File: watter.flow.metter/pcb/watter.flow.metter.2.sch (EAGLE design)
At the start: 19 parts, among them Q1 BC546A

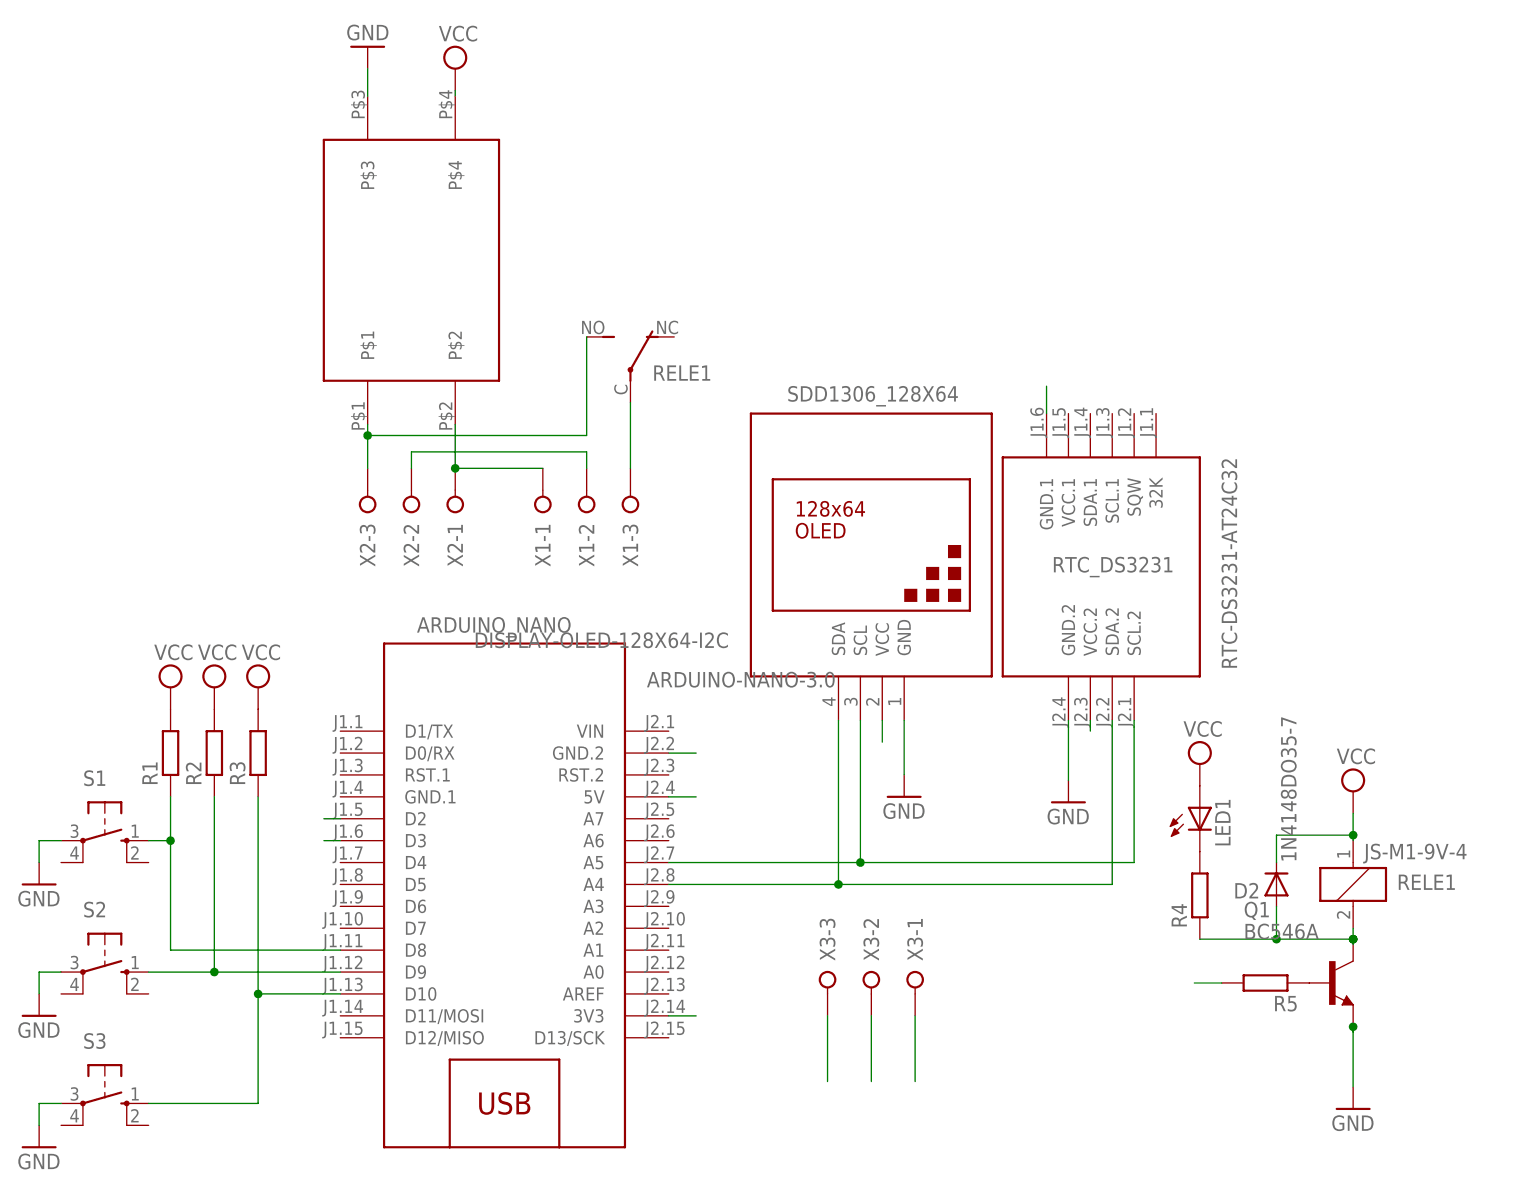
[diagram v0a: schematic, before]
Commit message: add terminal
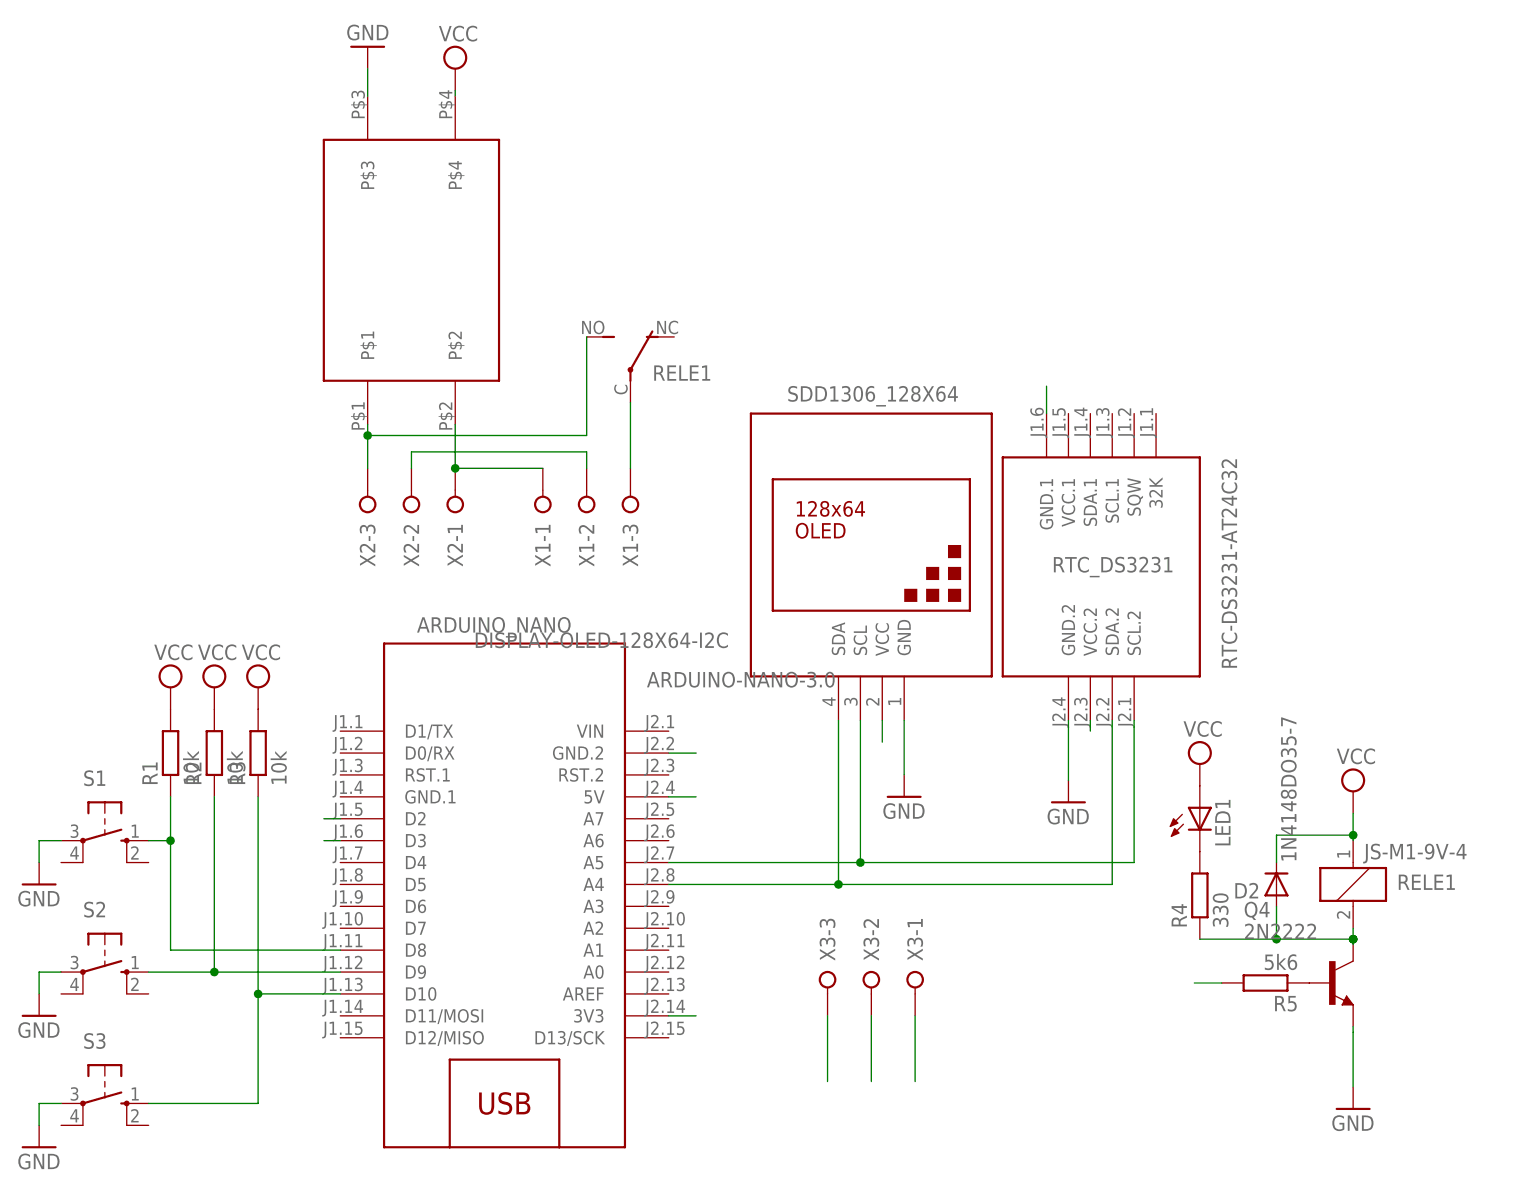
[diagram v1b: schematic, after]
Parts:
- removed Q1: BC546A, transistor-npn:BC546A
- added Q4: 2N2222, transistor-npn:2N5088
- R1, R2, R3: value (none) -> 10k
- R4: value (none) -> 330
- R5: value (none) -> 5k6
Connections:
- net GND: now also Q4.E; no longer Q1.E
- net N$41: now also Q4.C; no longer Q1.C
- net N$7: now also Q4.B; no longer Q1.B
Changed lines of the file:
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@@
 <?xml version="1.0" encoding="utf-8"?>
 <!DOCTYPE eagle SYSTEM "eagle.dtd">
-<eagle version="8.2.2">
+<eagle version="8.4.1">
 <drawing>
 <settings>
 <setting alwaysvectorfont="no"/>
+<setting keepoldvectorfont="yes"/>
 <setting verticaltext="up"/>
 </settings>
-<grid distance="0.1" unitdist="inch" unit="inch" style="lines" multiple="1" display="no" altdistance="0.01" altunitdist="inch" altunit="inch"/>
+<grid distance="0.05" unitdist="inch" unit="inch" style="lines" multiple="1" display="no" altdistance="0.01" altunitdist="inch" altunit="inch"/>
 <layers>
 <layer number="1" name="Top" color="4" fill="1" visible="no" active="no"/>
@@
 <part name="SUPPLY4" library="supply2" library_urn="urn:adsk.eagle:library:372" deviceset="VCC" device=""/>
 <part name="SUPPLY6" library="supply2" library_urn="urn:adsk.eagle:library:372" deviceset="VCC" device=""/>
-<part name="R1" library="rcl" library_urn="urn:adsk.eagle:library:334" deviceset="R-EU_" device="0207/10"/>
-<part name="R2" library="rcl" library_urn="urn:adsk.eagle:library:334" deviceset="R-EU_" device="0207/10"/>
-<part name="R3" library="rcl" library_urn="urn:adsk.eagle:library:334" deviceset="R-EU_" device="0207/10"/>
-<part name="Q1" library="transistor-npn" library_urn="urn:adsk.eagle:library:398" deviceset="BC546*" device="" technology="A"/>
+<part name="R1" library="rcl" library_urn="urn:adsk.eagle:library:334" deviceset="R-EU_" device="0207/10" value="10k"/>
+<part name="R2" library="rcl" library_urn="urn:adsk.eagle:library:334" deviceset="R-EU_" device="0207/10" value="10k"/>
+<part name="R3" library="rcl" library_urn="urn:adsk.eagle:library:334" deviceset="R-EU_" device="0207/10" value="10k"/>
 <part name="SUPPLY7" library="supply2" library_urn="urn:adsk.eagle:library:372" deviceset="VCC" device=""/>
 <part name="LED1" library="led" library_urn="urn:adsk.eagle:library:259" deviceset="LED" device="3MM"/>
-<part name="R4" library="rcl" library_urn="urn:adsk.eagle:library:334" deviceset="R-EU_" device="0207/10"/>
+<part name="R4" library="rcl" library_urn="urn:adsk.eagle:library:334" deviceset="R-EU_" device="0207/10" value="330"/>
 <part name="SDD1306_128X64" library="diy-modules" deviceset="DISPLAY-OLED-128X64-I2C" device=""/>
 <part name="X3" library="con-wago-508" library_urn="urn:adsk.eagle:library:196" deviceset="W237-3E" device=""/>
 <part name="RTC_DS3231" library="diy-modules" deviceset="RTC-DS3231-AT24C32" device=""/>
 <part name="U$6" library="diy-modules" deviceset="HLK-PM01" device=""/>
-<part name="R5" library="rcl" library_urn="urn:adsk.eagle:library:334" deviceset="R-EU_" device="0207/10"/>
+<part name="R5" library="rcl" library_urn="urn:adsk.eagle:library:334" deviceset="R-EU_" device="0207/10" value="5k6"/>
 <part name="D2" library="diode" library_urn="urn:adsk.eagle:library:210" deviceset="1N4148" device="DO35-7"/>
 <part name="ARDUINO_NANO" library="diy-modules" deviceset="ARDUINO-NANO-3.0" device=""/>
 <part name="X1" library="con-wago-508" library_urn="urn:adsk.eagle:library:196" deviceset="W237-3E" device=""/>
+<part name="Q4" library="transistor-npn" library_urn="urn:adsk.eagle:library:398" deviceset="2N5088" device="" package3d_urn="urn:adsk.eagle:package:28974/2" value="2N2222"/>
 </parts>
 <sheets>
@@
 <instance part="R2" gate="G$1" x="-25.4" y="66.04" rot="R90"/>
 <instance part="R3" gate="G$1" x="-20.32" y="66.04" rot="R90"/>
-<instance part="Q1" gate="G$1" x="104.14" y="39.37"/>
 <instance part="SUPPLY7" gate="G$1" x="88.9" y="64.77"/>
 <instance part="LED1" gate="G$1" x="88.9" y="59.69"/>
@@
 <instance part="X1" gate="-2" x="17.78" y="93.98" rot="R90"/>
 <instance part="X1" gate="-3" x="22.86" y="93.98" rot="R90"/>
+<instance part="Q4" gate="G$1" x="104.14" y="39.37"/>
 </instances>
 <busses>
@@
 <segment>
 <pinref part="GND13" gate="1" pin="GND"/>
-<wire x1="106.68" y1="27.305" x2="106.68" y2="34.29" width="0.1524" layer="91"/>
-<pinref part="Q1" gate="G$1" pin="E"/>
+<wire x1="106.68" y1="27.305" x2="106.68" y2="33.655" width="0.1524" layer="91"/>
 <wire x1="106.68" y1="34.29" x2="106.68" y2="33.655" width="0.1524" layer="91"/>
-<junction x="106.68" y="34.29"/>
+<pinref part="Q4" gate="G$1" pin="E"/>
 </segment>
 <segment>
@@
 <junction x="106.68" y="44.45"/>
 <pinref part="RELE1" gate="1" pin="2"/>
-<pinref part="Q1" gate="G$1" pin="C"/>
 <junction x="106.68" y="44.45"/>
 <pinref part="R4" gate="G$1" pin="1"/>
@@
 <junction x="97.79" y="44.45"/>
 <pinref part="D2" gate="G$1" pin="A"/>
+<pinref part="Q4" gate="G$1" pin="C"/>
 </segment>
 </net>
@@
 </segment>
 </net>
-<net name="N$7" class="0">
-<segment>
-<pinref part="Q1" gate="G$1" pin="B"/>
-<pinref part="R5" gate="G$1" pin="1"/>
-</segment>
-</net>
 <net name="N$3" class="0">
 <segment>
@@
 <wire x1="-2.54" y1="100.965" x2="17.78" y2="100.965" width="0.1524" layer="91"/>
 <wire x1="17.78" y1="100.965" x2="17.78" y2="99.06" width="0.1524" layer="91"/>
+</segment>
+</net>
+<net name="N$7" class="0">
+<segment>
+<pinref part="R5" gate="G$1" pin="1"/>
+<pinref part="Q4" gate="G$1" pin="B"/>
 </segment>
 </net>
@@
 <compatibility>
 <note version="8.2" severity="warning">
-Since Version 8.2, Eagle supports online libraries. The ids
+Since Version 8.2, EAGLE supports online libraries. The ids
 of those online libraries will not be understood (or retained)
 with this version.
 </note>
+<note version="8.3" severity="warning">
+Since Version 8.3, EAGLE supports URNs for individual library
+assets (packages, symbols, and devices). The URNs of those assets
+will not be understood (or retained) with this version.
+</note>
+<note version="8.3" severity="warning">
+Since Version 8.3, EAGLE supports the association of 3D packages
+with devices in libraries, schematics, and board files. Those 3D
+packages will not be understood (or retained) with this version.
+</note>
 </compatibility>
